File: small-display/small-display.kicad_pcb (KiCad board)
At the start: 4 copper layers, 43 x 62 mm, 44 parts, among them J1 2047110001, J2 Micro_SD_Card_Det, J5 F32D-1A7Y1-21040, U1 TPD4EUSB30, U2 74LVC1G07SE-7, U3 RT9742GGJ5, U4 PAM2804AAB010, U5 USB2412-DZK, U6 NLVVHC1G04DFT1G, U7 M24M01-DFDW6TP, Y1 ECS-240-8-33-AGN-TR

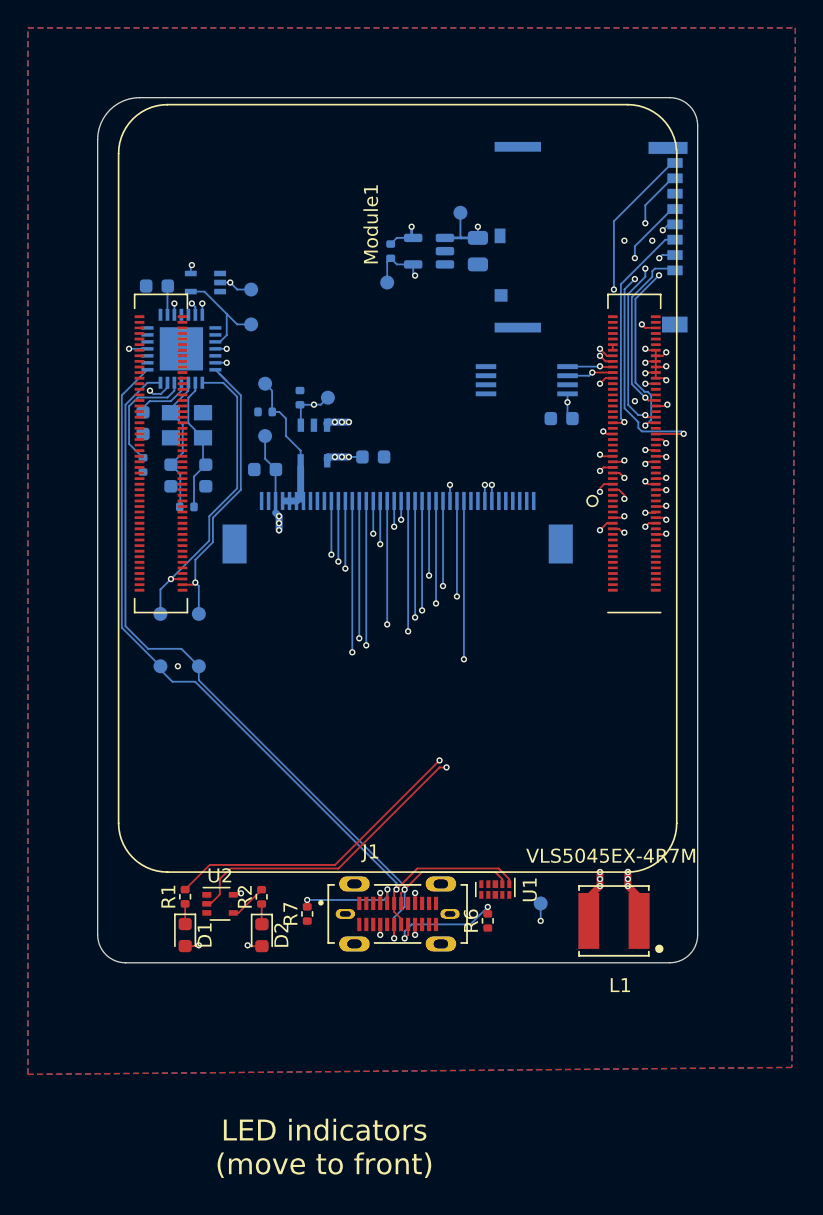
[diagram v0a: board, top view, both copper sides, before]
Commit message: More or less complete except for DRC.
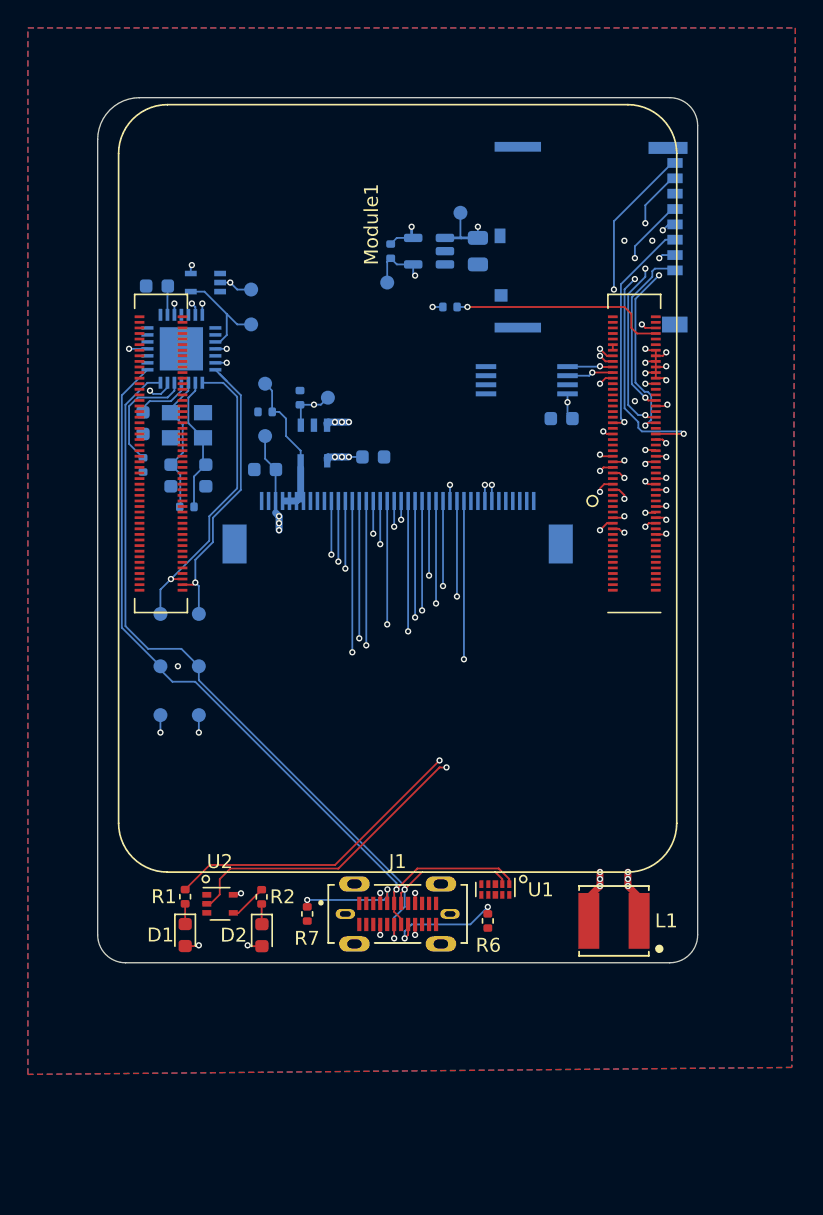
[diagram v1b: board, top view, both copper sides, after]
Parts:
- added R10: 10k, Resistor_SMD:R_0402_1005Metric, B.Cu at (25.2, 15.0)
- added TP13: TestPoint, TestPoint:TestPoint_Pad_D1.0mm, B.Cu at (4.50, 44.2)
- moved TP3 28.0 mm to (7.25, 44.2)
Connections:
- Module1 pad 101: USBOTG_ID -> GND
- Module1 pad 102: /PCIE_CLK_nREQ -> unconnected-(Module1-Pad102)
- Module1 pad 109: PCIE_nRST -> unconnected-(Module1-Pad109)
- Module1 pad 11: TRD2_P -> unconnected-(Module1-Pad11)
- Module1 pad 110: /PCIE_CLK_P -> unconnected-(Module1-Pad110)
- Module1 pad 111: TV_OUT -> unconnected-(Module1-Pad111)
- Module1 pad 112: /PCIE_CLK_N -> unconnected-(Module1-Pad112)
- Module1 pad 115: CAM1_D0_N -> unconnected-(Module1-Pad115)
- Module1 pad 116: /PCIE_RX_P -> unconnected-(Module1-Pad116)
- Module1 pad 117: CAM1_D0_P -> unconnected-(Module1-Pad117)
- Module1 pad 118: /PCIE_RX_N -> unconnected-(Module1-Pad118)
- Module1 pad 121: CAM1_D1_N -> unconnected-(Module1-Pad121)
- Module1 pad 122: /PCIE_TX_P -> unconnected-(Module1-Pad122)
- Module1 pad 123: CAM1_D1_P -> unconnected-(Module1-Pad123)
- Module1 pad 124: /PCIE_TX_N -> unconnected-(Module1-Pad124)
- Module1 pad 127: CAM1_C_N -> unconnected-(Module1-Pad127)
- Module1 pad 128: /CAM0_D0_N -> unconnected-(Module1-Pad128)
- Module1 pad 129: CAM1_C_P -> unconnected-(Module1-Pad129)
- Module1 pad 130: /CAM0_D0_P -> unconnected-(Module1-Pad130)
- Module1 pad 133: CAM1_D2_N -> unconnected-(Module1-Pad133)
- Module1 pad 134: /CAM0_D1_N -> unconnected-(Module1-Pad134)
- Module1 pad 135: CAM1_D2_P -> unconnected-(Module1-Pad135)
- Module1 pad 136: /CAM0_D1_P -> unconnected-(Module1-Pad136)
- Module1 pad 139: CAM1_D3_N -> unconnected-(Module1-Pad139)
- Module1 pad 140: /CAM0_C_N -> unconnected-(Module1-Pad140)
- Module1 pad 141: CAM1_D3_P -> unconnected-(Module1-Pad141)
- Module1 pad 142: /CAM0_C_P -> unconnected-(Module1-Pad142)
- Module1 pad 143: HDMI1_HOTPLUG -> unconnected-(Module1-Pad143)
- Module1 pad 145: HDMI1_SDA -> unconnected-(Module1-Pad145)
- Module1 pad 146: /HDMI1_D2_P -> unconnected-(Module1-Pad146)
- Module1 pad 147: HDMI1_SCL -> unconnected-(Module1-Pad147)
- Module1 pad 148: /HDMI1_D2_N -> unconnected-(Module1-Pad148)
- Module1 pad 149: HDMI1_CEC -> unconnected-(Module1-Pad149)
- Module1 pad 15: ETH_LEDY -> unconnected-(Module1-Pad15)
- Module1 pad 151: HDMI0_CEC -> unconnected-(Module1-Pad151)
- Module1 pad 152: /HDMI1_D1_P -> unconnected-(Module1-Pad152)
- Module1 pad 153: HDMI0_HOTPLUG -> unconnected-(Module1-Pad153)
- Module1 pad 154: /HDMI1_D1_N -> unconnected-(Module1-Pad154)
- Module1 pad 157: DSI0_D0_N -> unconnected-(Module1-Pad157)
- Module1 pad 158: /HDMI1_D0_P -> unconnected-(Module1-Pad158)
- Module1 pad 159: DSI0_D0_P -> unconnected-(Module1-Pad159)
- Module1 pad 160: /HDMI1_D0_N -> unconnected-(Module1-Pad160)
- Module1 pad 163: DSI0_D1_N -> unconnected-(Module1-Pad163)
- Module1 pad 164: /HDMI1_CK_P -> unconnected-(Module1-Pad164)
- Module1 pad 165: DSI0_D1_P -> unconnected-(Module1-Pad165)
- Module1 pad 166: /HDMI1_CK_N -> unconnected-(Module1-Pad166)
- Module1 pad 169: DSI0_C_N -> unconnected-(Module1-Pad169)
- Module1 pad 17: ETH_LEDG -> unconnected-(Module1-Pad17)
- Module1 pad 170: /HDMI0_D2_P -> unconnected-(Module1-Pad170)
- Module1 pad 171: DSI0_C_P -> unconnected-(Module1-Pad171)
- Module1 pad 172: /HDMI0_D2_N -> unconnected-(Module1-Pad172)
- Module1 pad 175: DSI1_D0_N -> unconnected-(Module1-Pad175)
- Module1 pad 176: /HDMI0_D1_P -> unconnected-(Module1-Pad176)
- Module1 pad 177: DSI1_D0_P -> unconnected-(Module1-Pad177)
- Module1 pad 178: /HDMI0_D1_N -> unconnected-(Module1-Pad178)
- Module1 pad 181: DSI1_D1_N -> unconnected-(Module1-Pad181)
- Module1 pad 182: /HDMI0_D0_P -> unconnected-(Module1-Pad182)
- Module1 pad 183: DSI1_D1_P -> unconnected-(Module1-Pad183)
- Module1 pad 184: /HDMI0_D0_N -> unconnected-(Module1-Pad184)
- Module1 pad 187: DSI1_C_N -> unconnected-(Module1-Pad187)
- Module1 pad 188: /HDMI0_CK_P -> unconnected-(Module1-Pad188)
- Module1 pad 189: DSI1_C_P -> unconnected-(Module1-Pad189)
- Module1 pad 190: /HDMI0_CK_N -> unconnected-(Module1-Pad190)
- Module1 pad 193: DSI1_D2_N -> unconnected-(Module1-Pad193)
- Module1 pad 194: /DSI1_D3_N -> unconnected-(Module1-Pad194)
- Module1 pad 195: DSI1_D2_P -> unconnected-(Module1-Pad195)
- Module1 pad 196: /DSI1_D3_P -> unconnected-(Module1-Pad196)
- Module1 pad 199: HDMI0_SDA -> unconnected-(Module1-Pad199)
- Module1 pad 200: /HDMI0_SCL -> unconnected-(Module1-Pad200)
- Module1 pad 3: TRD3_P -> unconnected-(Module1-Pad3)
- Module1 pad 30: GPIO6 -> unconnected-(Module1-Pad30)
- Module1 pad 33: GND -> unconnected-(Module1-Pad33)
- Module1 pad 34: GPIO5 -> unconnected-(Module1-Pad34)
- Module1 pad 35: ID_SC -> unconnected-(Module1-Pad35)
- Module1 pad 36: ID_SD -> unconnected-(Module1-Pad36)
- Module1 pad 45: GPIO24 -> unconnected-(Module1-Pad45)
- Module1 pad 5: TRD3_N -> unconnected-(Module1-Pad5)
- Module1 pad 54: GPIO4 -> unconnected-(Module1-Pad54)
- Module1 pad 56: GPIO3 -> unconnected-(Module1-Pad56)
- Module1 pad 9: TRD2_N -> unconnected-(Module1-Pad9)
- Module1 pad 92: RUN_PG -> unconnected-(Module1-Pad92)
- Module1 pad 93: unconnected-(Module1-Pad93) -> /nRPIBOOT
- Module1 pad 94: AIN1 -> unconnected-(Module1-Pad94)
- Module1 pad 96: AIN0 -> unconnected-(Module1-Pad96)
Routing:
- net /nRPIBOOT: track 0.00 -> 15.6 mm, vias 0 -> 1
- net +3.3V: track 21.0 -> 23.0 mm, vias 18 -> 20
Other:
- board text removed: "LED indicators (move to front)"
